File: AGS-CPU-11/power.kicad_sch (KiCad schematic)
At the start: 63 parts, among them Q3 2SK3663, Q5 2SJ647, T1 GameBoy_Transformer_AGS, U4 S6403/9753, U7 ???

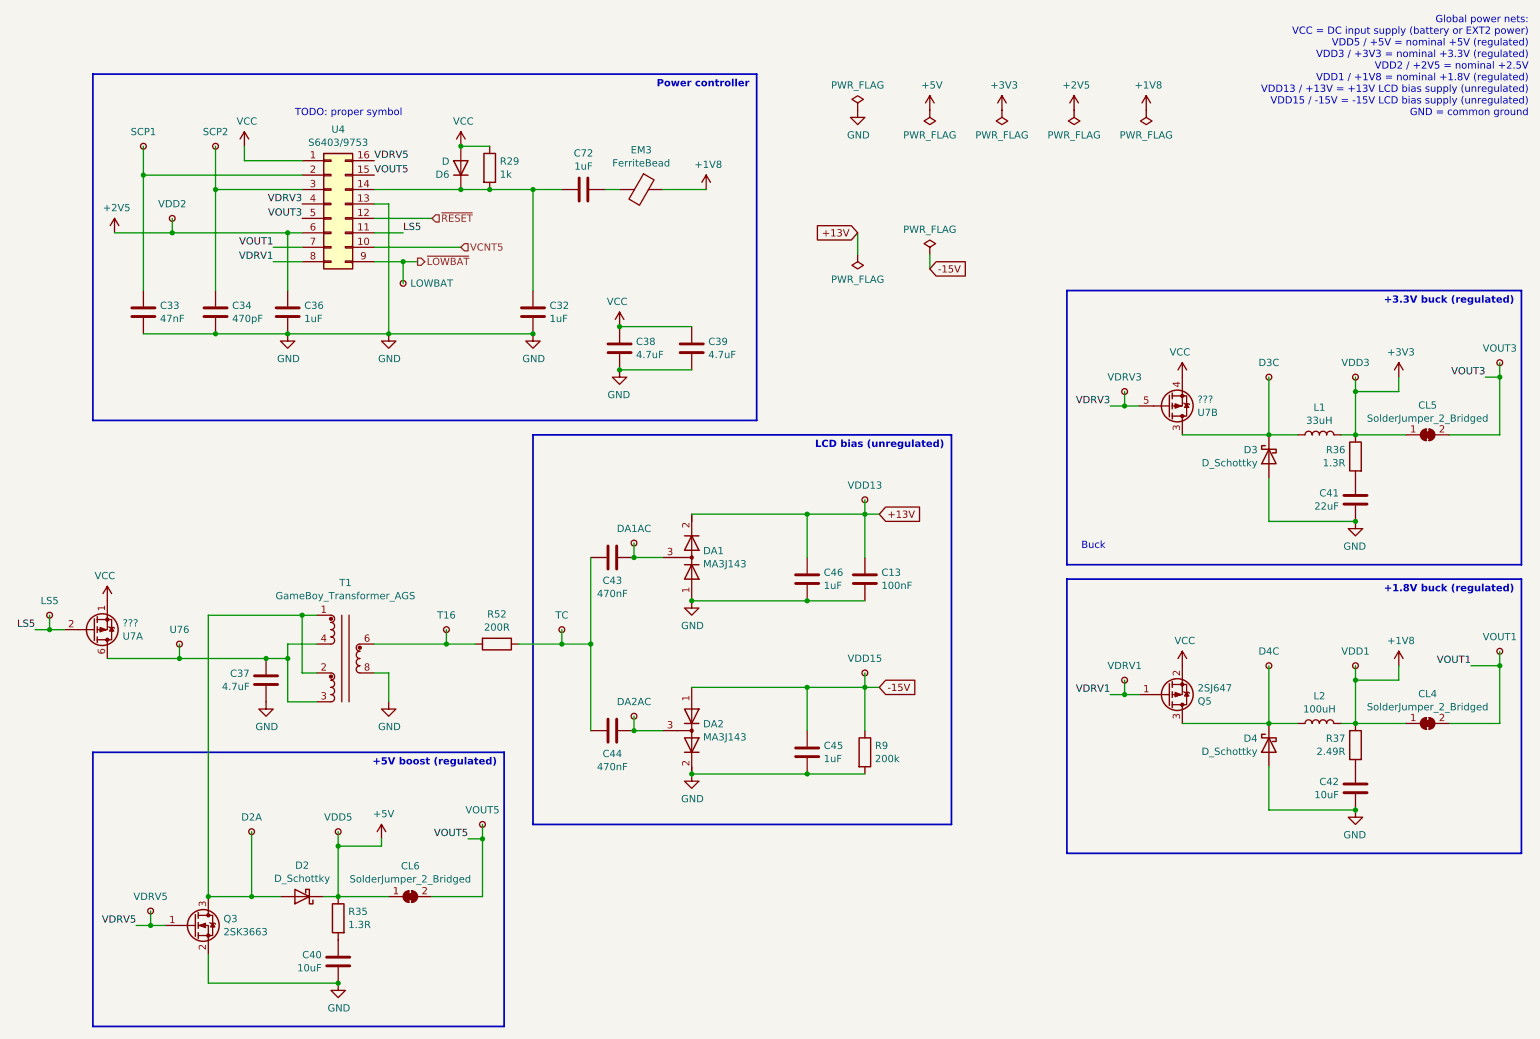
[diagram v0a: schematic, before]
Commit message: Update to latest KiCad
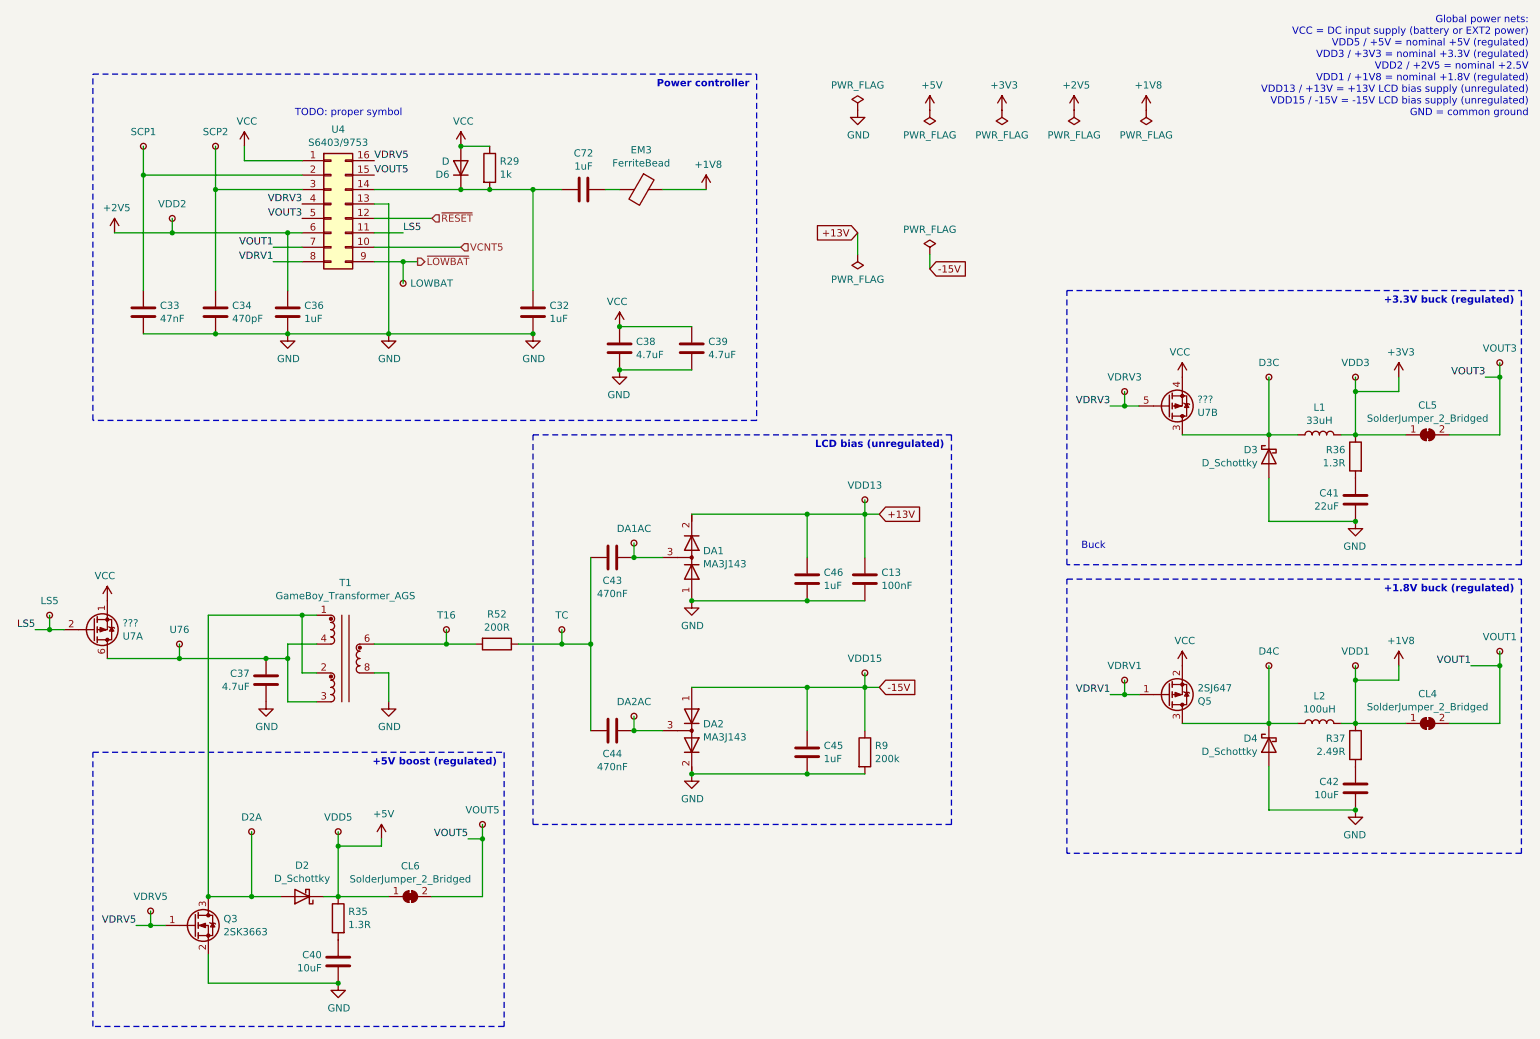
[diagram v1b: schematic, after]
